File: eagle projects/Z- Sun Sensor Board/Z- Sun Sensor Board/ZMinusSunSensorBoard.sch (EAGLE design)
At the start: 189 parts, among them J2 HIROSE_FH19C-6S-0.5SH(10), J3 HIROSE_FH19C-6S-0.5SH(10), J4 HIROSE_FH19C-6S-0.5SH(10), J5 HIROSE_FH19C-6S-0.5SH(10), U1 ADS7841E_2K5, U13 ADS7841E_2K5, U15 TLV9051IDCKR, U19 TLV9051IDCKR, U2 ADS7841E_2K5, U21 TLV9051IDCKR, U23 TLV9051IDCKR, U24 TLV9051IDCKR, U25 ADS7841E_2K5, U26 TLV9051IDCKR, U27 ADS7841E_2K5, U28 TLV9051IDCKR, U29 TLV9051IDCKR, U3 TLV9051IDCKR, U30 TLV9051IDCKR, U31 TLV9051IDCKR, U32 TLV9051IDCKR, U4 LM20BIM7X_NOPB, U6 TLV9051IDCKR, U8 TLV9051IDCKR, U9 TLV9051IDCKR

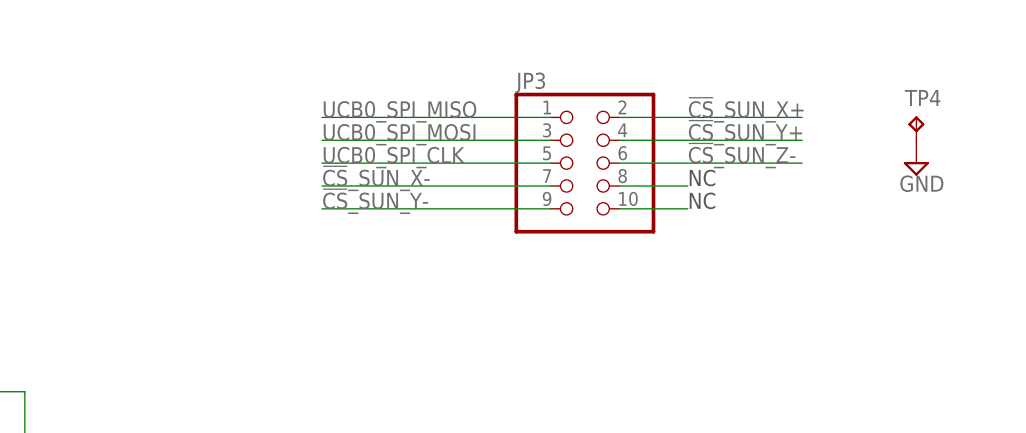
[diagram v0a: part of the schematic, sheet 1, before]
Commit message: Sanity check
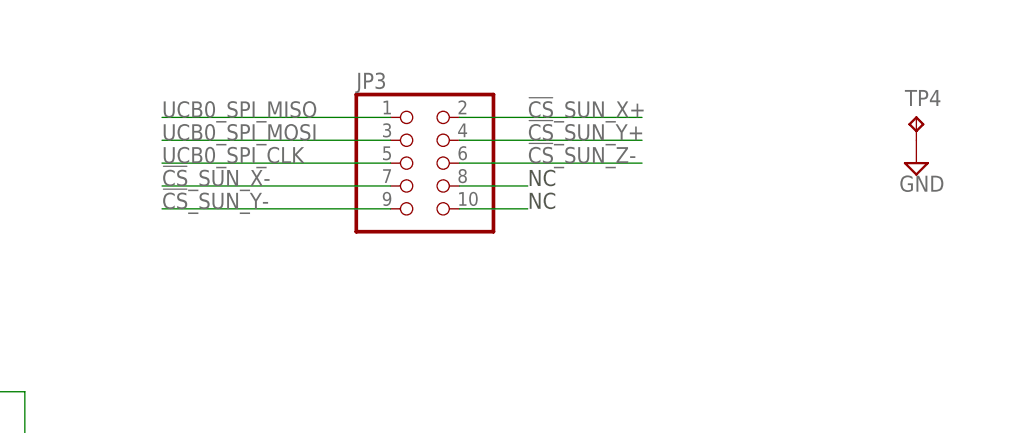
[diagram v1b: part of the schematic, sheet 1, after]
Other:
- moved on the sheet: JP3
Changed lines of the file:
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@@
 <schematic_group name="POWER5"/>
 <schematic_group name="POWER"/>
+<schematic_group name="MSP430_BOARD_SENSOR"/>
 </groups>
 <parts>
@@
 <text x="10.16" y="25.4" size="1.778" layer="97">Custom machine sun sensor mount for Z- face
 photodiodes mechanically to board</text>
-<text x="228.6" y="185.42" size="1.778" layer="97">NC</text>
-<text x="228.6" y="182.88" size="1.778" layer="97">NC</text>
+<text x="210.82" y="185.42" size="1.778" layer="97" grouprefs="MSP430_BOARD_SENSOR">NC</text>
+<text x="210.82" y="182.88" size="1.778" layer="97" grouprefs="MSP430_BOARD_SENSOR">NC</text>
 </plain>
 <instances>
@@
 <attribute name="VALUE" x="36.83" y="152.4" size="1.778" layer="96"/>
 </instance>
-<instance part="JP3" gate="A" x="215.9" y="187.96" smashed="yes">
-<attribute name="NAME" x="209.55" y="196.215" size="1.778" layer="95"/>
-<attribute name="VALUE" x="209.55" y="177.8" size="1.778" layer="96"/>
+<instance part="JP3" gate="A" x="198.12" y="187.96" smashed="yes" grouprefs="MSP430_BOARD_SENSOR">
+<attribute name="NAME" x="191.77" y="196.215" size="1.778" layer="95"/>
+<attribute name="VALUE" x="191.77" y="177.8" size="1.778" layer="96"/>
 </instance>
 <instance part="LED1" gate="G$1" x="12.7" y="157.48" smashed="yes" grouprefs="POWER">
@@
 <segment>
 <pinref part="JP3" gate="A" pin="3"/>
-<wire x1="213.36" y1="190.5" x2="187.96" y2="190.5" width="0.1524" layer="91"/>
-<label x="187.96" y="190.5" size="1.778" layer="95"/>
+<wire x1="195.58" y1="190.5" x2="170.18" y2="190.5" width="0.1524" layer="91" grouprefs="MSP430_BOARD_SENSOR"/>
+<label x="170.18" y="190.5" size="1.778" layer="95" grouprefs="MSP430_BOARD_SENSOR"/>
 </segment>
 </net>
@@
 <segment>
 <pinref part="JP3" gate="A" pin="5"/>
-<wire x1="213.36" y1="187.96" x2="187.96" y2="187.96" width="0.1524" layer="91"/>
-<label x="187.96" y="187.96" size="1.778" layer="95"/>
+<wire x1="195.58" y1="187.96" x2="170.18" y2="187.96" width="0.1524" layer="91" grouprefs="MSP430_BOARD_SENSOR"/>
+<label x="170.18" y="187.96" size="1.778" layer="95" grouprefs="MSP430_BOARD_SENSOR"/>
 </segment>
 </net>
@@
 <segment>
 <pinref part="JP3" gate="A" pin="1"/>
-<wire x1="213.36" y1="193.04" x2="187.96" y2="193.04" width="0.1524" layer="91"/>
-<label x="187.96" y="193.04" size="1.778" layer="95"/>
+<wire x1="195.58" y1="193.04" x2="170.18" y2="193.04" width="0.1524" layer="91" grouprefs="MSP430_BOARD_SENSOR"/>
+<label x="170.18" y="193.04" size="1.778" layer="95" grouprefs="MSP430_BOARD_SENSOR"/>
 </segment>
 </net>
@@
 <segment>
 <pinref part="JP3" gate="A" pin="2"/>
-<wire x1="220.98" y1="193.04" x2="241.3" y2="193.04" width="0.1524" layer="91"/>
-<label x="228.6" y="193.04" size="1.778" layer="95"/>
+<wire x1="203.2" y1="193.04" x2="223.52" y2="193.04" width="0.1524" layer="91" grouprefs="MSP430_BOARD_SENSOR"/>
+<label x="210.82" y="193.04" size="1.778" layer="95" grouprefs="MSP430_BOARD_SENSOR"/>
 </segment>
 </net>
@@
 <segment>
 <pinref part="JP3" gate="A" pin="7"/>
-<wire x1="213.36" y1="185.42" x2="187.96" y2="185.42" width="0.1524" layer="91"/>
-<label x="187.96" y="185.42" size="1.778" layer="95"/>
+<wire x1="195.58" y1="185.42" x2="170.18" y2="185.42" width="0.1524" layer="91" grouprefs="MSP430_BOARD_SENSOR"/>
+<label x="170.18" y="185.42" size="1.778" layer="95" grouprefs="MSP430_BOARD_SENSOR"/>
 </segment>
 </net>
@@
 <segment>
 <pinref part="JP3" gate="A" pin="4"/>
-<wire x1="220.98" y1="190.5" x2="241.3" y2="190.5" width="0.1524" layer="91"/>
-<label x="228.6" y="190.5" size="1.778" layer="95"/>
+<wire x1="203.2" y1="190.5" x2="223.52" y2="190.5" width="0.1524" layer="91" grouprefs="MSP430_BOARD_SENSOR"/>
+<label x="210.82" y="190.5" size="1.778" layer="95" grouprefs="MSP430_BOARD_SENSOR"/>
 </segment>
 </net>
@@
 <segment>
 <pinref part="JP3" gate="A" pin="9"/>
-<wire x1="213.36" y1="182.88" x2="187.96" y2="182.88" width="0.1524" layer="91"/>
-<label x="187.96" y="182.88" size="1.778" layer="95"/>
+<wire x1="195.58" y1="182.88" x2="170.18" y2="182.88" width="0.1524" layer="91" grouprefs="MSP430_BOARD_SENSOR"/>
+<label x="170.18" y="182.88" size="1.778" layer="95" grouprefs="MSP430_BOARD_SENSOR"/>
 </segment>
 </net>
@@
 <segment>
 <pinref part="JP3" gate="A" pin="6"/>
-<wire x1="220.98" y1="187.96" x2="241.3" y2="187.96" width="0.1524" layer="91"/>
-<label x="228.6" y="187.96" size="1.778" layer="95"/>
+<wire x1="203.2" y1="187.96" x2="223.52" y2="187.96" width="0.1524" layer="91" grouprefs="MSP430_BOARD_SENSOR"/>
+<label x="210.82" y="187.96" size="1.778" layer="95" grouprefs="MSP430_BOARD_SENSOR"/>
 </segment>
 </net>
@@
 <segment>
 <pinref part="JP3" gate="A" pin="8"/>
-<wire x1="228.6" y1="185.42" x2="220.98" y2="185.42" width="0.1524" layer="91"/>
+<wire x1="210.82" y1="185.42" x2="203.2" y2="185.42" width="0.1524" layer="91" grouprefs="MSP430_BOARD_SENSOR"/>
 </segment>
 </net>
@@
 <segment>
 <pinref part="JP3" gate="A" pin="10"/>
-<wire x1="220.98" y1="182.88" x2="228.6" y2="182.88" width="0.1524" layer="91"/>
-</segment>
-</net>
+<wire x1="203.2" y1="182.88" x2="210.82" y2="182.88" width="0.1524" layer="91" grouprefs="MSP430_BOARD_SENSOR"/>
+</segment>
+</net>
